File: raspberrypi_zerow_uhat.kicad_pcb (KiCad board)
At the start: 2 copper layers, 65 x 30 mm, 14 parts, among them IC1 3006, J1 GPIO_CONNECTOR, J3 Mic connector

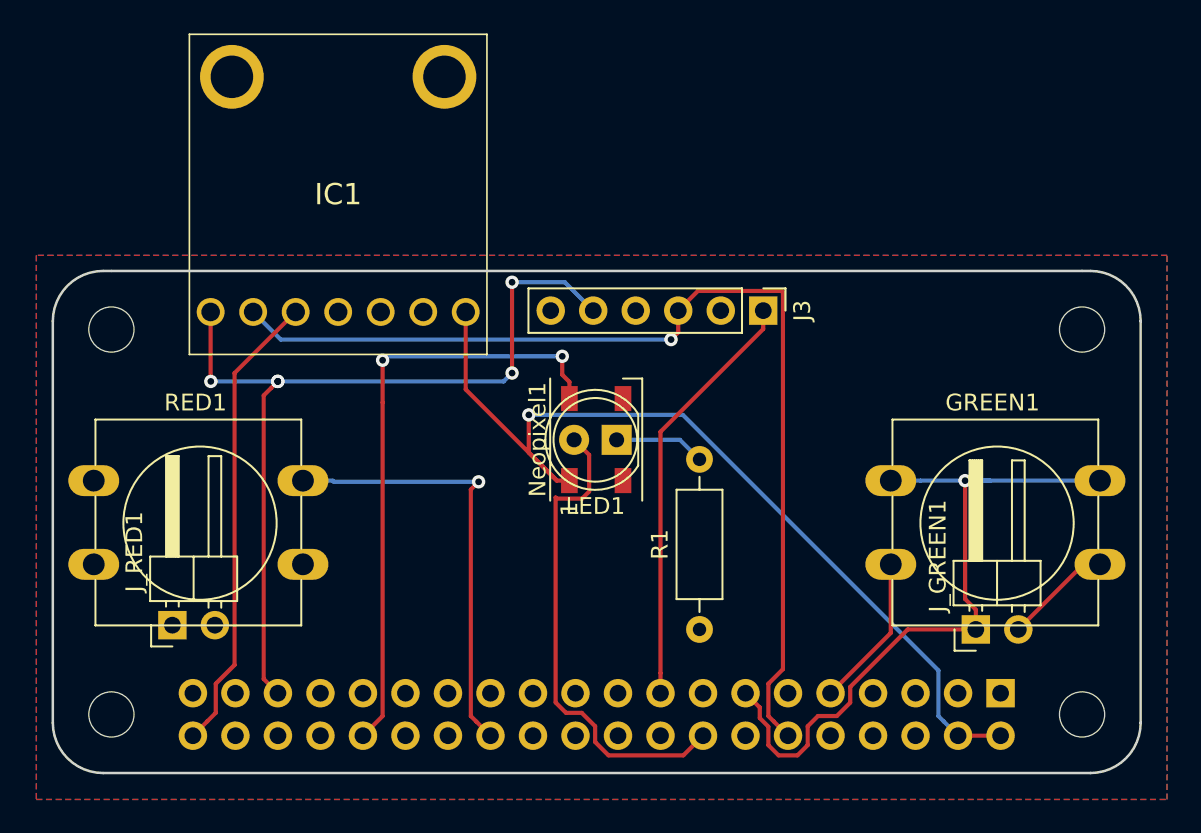
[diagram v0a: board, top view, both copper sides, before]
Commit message: v1.0
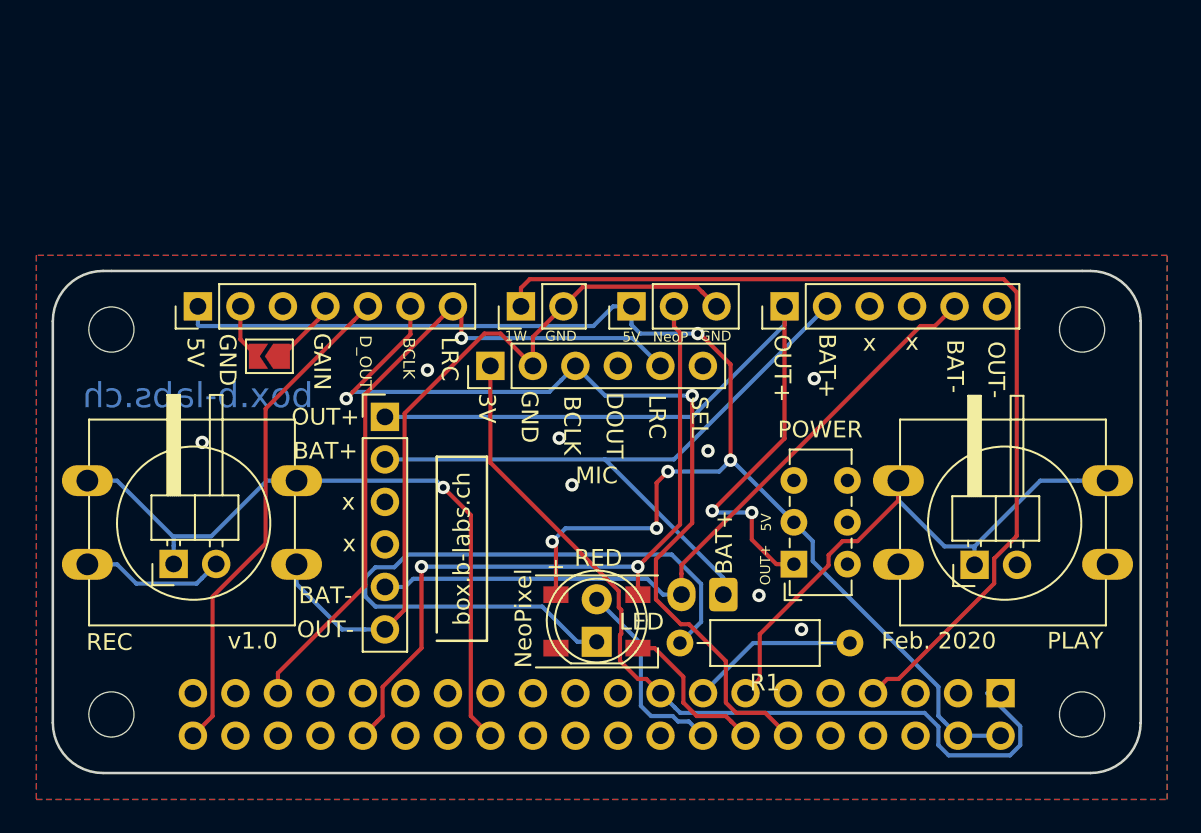
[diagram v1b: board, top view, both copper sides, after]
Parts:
- removed IC1: 3006, 3006:3006
- added J2: Amp connector, Connector_PinHeader_2.54mm:PinHeader_1x07_P2.54mm_Vertical, F.Cu at (103.8, 95.6)
- added J4: OneWire, Connector_PinHeader_2.54mm:PinHeader_1x02_P2.54mm_Vertical, F.Cu at (123.1, 95.6)
- added J5: Neopixel connector, Connector_PinHeader_2.54mm:PinHeader_1x03_P2.54mm_Vertical, F.Cu at (129.7, 95.6)
- added J6: Battery, Connector_JST:JST_EH_S2B-EH_1x02_P2.50mm_Horizontal, B.Cu at (135.2, 112.8)
- added J7: Voltage Regulator Option A, Connector_PinHeader_2.54mm:PinHeader_1x06_P2.54mm_Vertical, F.Cu at (114.9, 102.2)
- added J8: Voltage Regulator Option B, Connector_PinHeader_2.54mm:PinHeader_1x06_P2.54mm_Vertical, F.Cu at (138.8, 95.6)
- added JP1: GainGND, Jumper:SolderJumper-2_P1.3mm_Open_TrianglePad1.0x1.5mm, F.Cu at (108.0, 98.6)
- added SW1: POWER, Button_Switch_THT:SW_E-Switch_EG1271_DPDT, F.Cu at (139.4, 111.0)
- moved J3 16.6 mm to (121.2, 99.1), turned to 90 degrees
- moved LED1 12.1 mm to (127.6, 115.6), turned to 90 degrees
- moved Neopixel1 10.9 mm to (127.6, 114.4), turned to 0 degrees
- moved R1 9.03 mm to (142.7, 115.7), turned to 180 degrees
- moved J_GREEN1 3.86 mm to (150.2, 111.0)
- moved J_RED1 3.66 mm to (102.3, 111.0)
- moved GREEN1 0.45 mm to (145.6, 106.0)
- moved RED1 0.38 mm to (97.2, 106.0)
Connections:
- net Net-(J3-Pad6) renamed SEL
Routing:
- net ONE_WIRE: track 0.00 -> 59.2 mm
- net GND: track 15.7 -> 67.4 mm, vias 0 -> 8
- net OUT+: track 0.00 -> 48.4 mm, vias 0 -> 2
- net BAT-: track 0.00 -> 43.1 mm
- net BAT+: track 0.00 -> 41.2 mm
- net Net-(LED1-Pad1): track 5.44 -> 41.5 mm
- net +5V: track 55.4 -> 83.4 mm, vias 2 -> 5
- net +3V3: track 25.4 -> 52.8 mm
- net RED_LED: track 29.1 -> 11.9 mm
- net RED_SWITCH: track 26.4 -> 41.9 mm
- net LRC: track 52.8 -> 42.1 mm, vias 5 -> 1
- net GREEN_LED: track 0.00 -> 10.0 mm
- net GREEN_SWITCH: track 43.9 -> 34.6 mm, vias 1 -> 0
- net BCLK: track 61.7 -> 55.1 mm, vias 1 -> 2
- net NEOPIXEL_DATA: track 36.5 -> 42.9 mm
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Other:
- board text added: "+"
- board text added: "1W"
- board text added: "3V"
- board text added: "5V"
- board text added: "BAT+"
- board text added: "BAT-"
- board text added: "BATTERY"
- board text added: "BCLK"
- board text added: "DOUT"
- board text added: "D_OUT"
- board text added: "Feb. 2020"
- board text added: "GAIN"
- board text added: "GND"
- board text added: "GREEN"
- board text added: "LED"
- board text added: "LRC"
- board text added: "MIC"
- board text added: "NeoP"
- board text added: "NeoPixel"
- board text added: "OUT+"
- board text added: "OUT-"
- board text added: "PLAY"
- board text added: "POWER"
- board text added: "REC"
- board text added: "RED"
- board text added: "SD"
- board text added: "SEL"
- board text added: "box.b-labs.ch"
- board text added: "v1.0"
- board text added: "x"
- board text removed: "Board dimensions are on Cmts (Comments) layer. Deselect it in Layers Manager to make them invisible. GPIO connector nets are not connected, these will get updated as per your schematic/netlist."
